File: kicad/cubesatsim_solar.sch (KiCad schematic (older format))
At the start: 23 parts, among them J1 Sensor Inputs, J10 INA219 Sensor Board, J11 INA219 Sensor Board, J12 INA219 Sensor Board, J13 3.5mm TRS Audio Jack with 2 S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, J14 RBF connector, J2 Battery In/Out, J3 Vdc In, J4 Vout to MoPOWER, J5 RBF Switch, J6 Expansion Interface, J7 INA219 Sensor Board, J8 INA219 Sensor Board, J9 INA219 Sensor Board, P3 Raspberry Pi GPIO Connector, U1 Variable Boost Converter Modu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

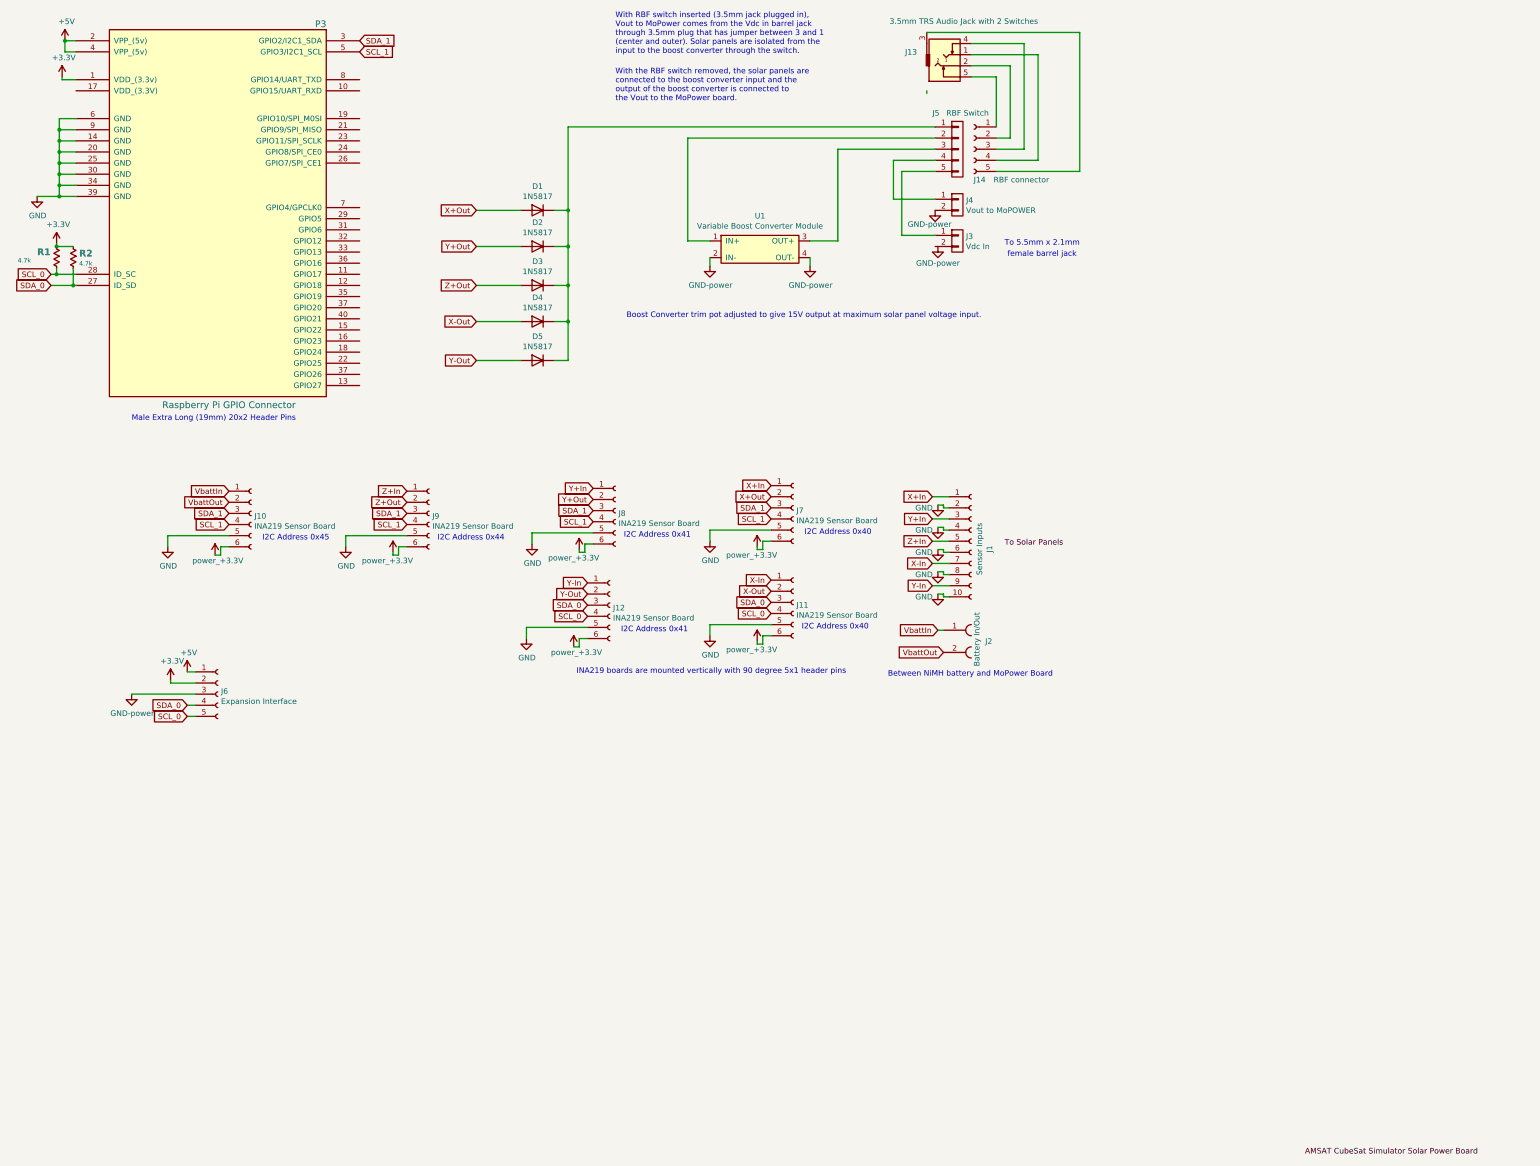
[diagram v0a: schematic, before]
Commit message: vB2 PCB Submitted to PCB Way
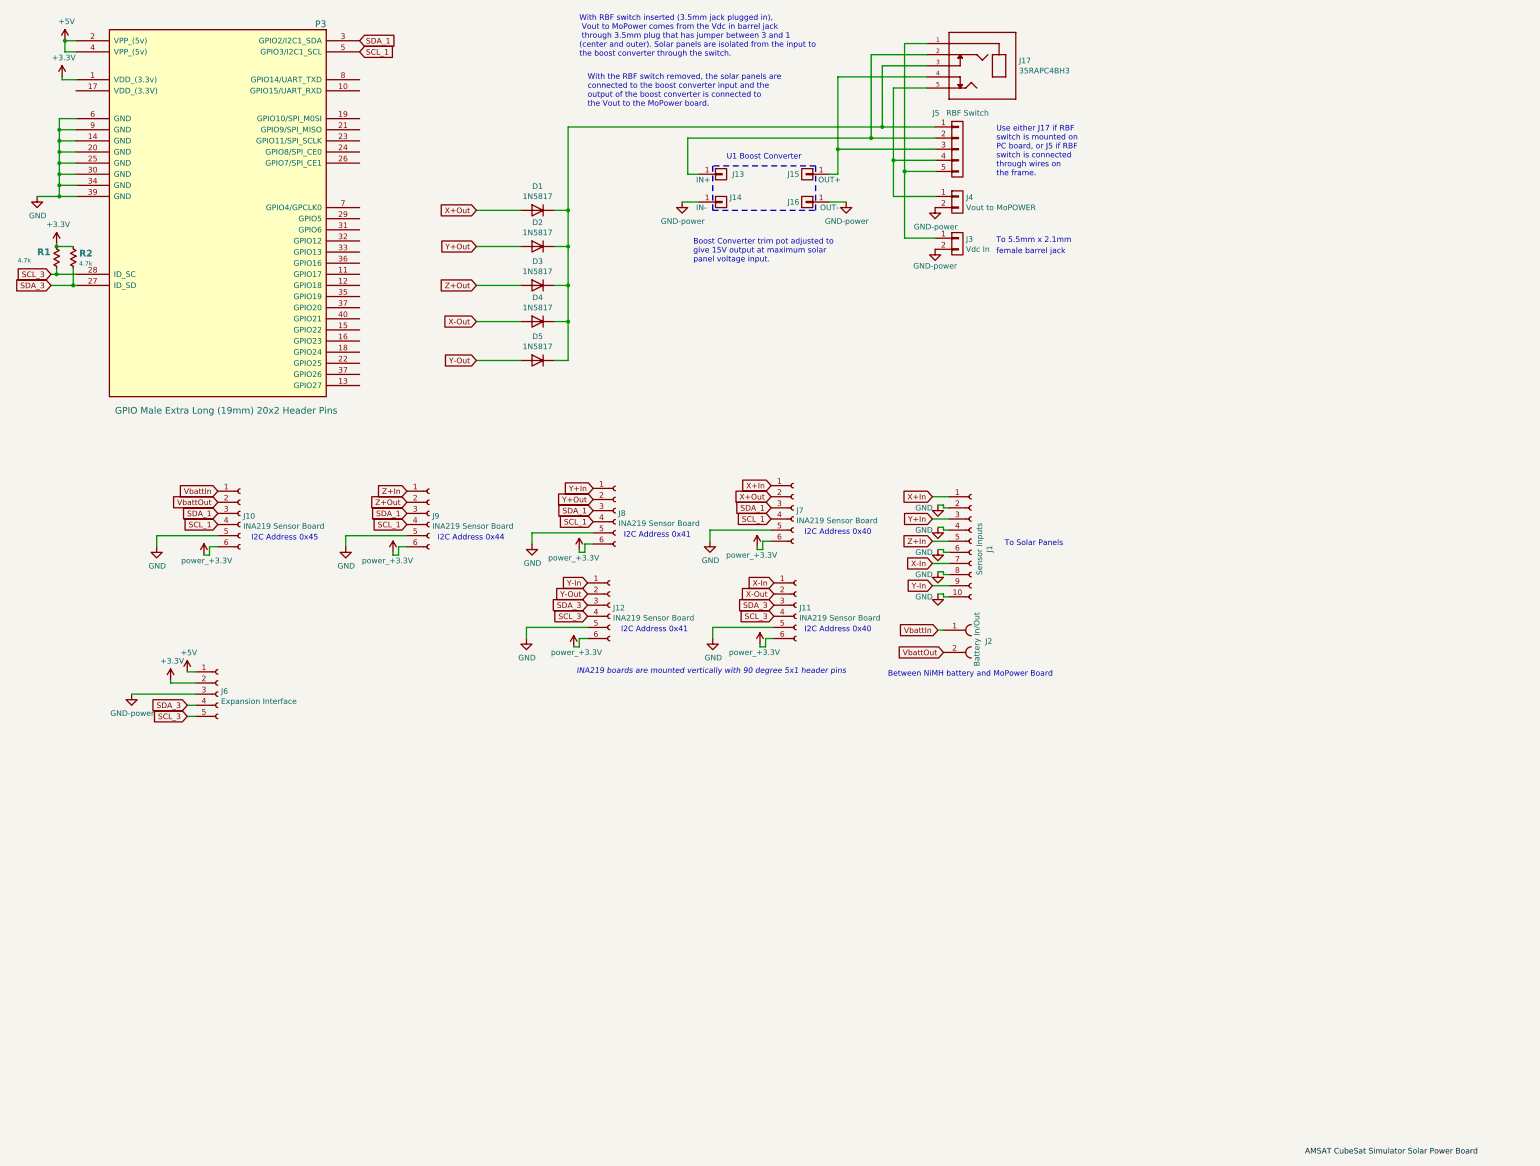
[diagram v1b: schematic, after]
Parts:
- removed J13: 3.5mm TRS Audio Jack with 2 Switches, symbol pihat_template-rescue:Audio-Jack-3_2Switches-conn2
- removed J14: RBF connector, symbol pihat_template-rescue:Conn_01x05_Female-Connector
- removed U1: Variable Boost Converter Module, symbol pihat_template-rescue:BoostConverter-New_Library
- added J13: IN+, Connector_PinSocket_2.54mm:PinSocket_1x01_P2.54mm_Vertical, symbol pihat_template-rescue:CONN_01X01-conn2
- added J14: IN-, Connector_PinSocket_2.54mm:PinSocket_1x01_P2.54mm_Vertical, symbol pihat_template-rescue:CONN_01X01-conn2
- added J15: OUT+, Connector_PinSocket_2.54mm:PinSocket_1x01_P2.54mm_Vertical, symbol pihat_template-rescue:CONN_01X01-conn2
- added J16: OUT-, Connector_PinSocket_2.54mm:PinSocket_1x01_P2.54mm_Vertical, symbol pihat_template-rescue:CONN_01X01-conn2
- added J17: 35RAPC4BH3, 35RAPC4BH3:SWITCHCRAFT_35RAPC4BH3, symbol 35RAPC4BH3:35RAPC4BH3
- J3, J4: footprint Connector_PinHeader_2.54mm:PinHeader_1x02_P2.54mm_Vertical -> Connector_Wire:SolderWirePad_1x02_P3.81mm_Drill1.2mm
- P3: value Raspberry Pi GPIO Connector -> GPIO Male Extra Long (19mm) 20x2 Header Pins; footprint w_conn_strip:vasch_strip_20x2 -> Connector_PinHeader_2.54mm:PinHeader_2x20_P2.54mm_Vertical
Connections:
- net GND: now also J3.2 (P2), J14.1 (P1), J16.1 (P1)
- net at D1.1 (K), D2.1 (K), D3.1 (K)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: now also J17.3
- net at J5.2 (P2): now also J13.1 (P1), J17.2
- net at J5.3 (P3): now also J15.1 (P1), J17.4
- net at J4.1 (P1), J5.4 (P4): now also J17.5
- net at J3.1 (P1), J5.5 (P5): now also J17.1
- net SCL_0 renamed SCL_3
- net SDA_0 renamed SDA_3
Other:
- note added: "Boost Converter trim pot adjusted to \ngive 15V output at maximum solar \npanel voltage input."
- note added: "To Solar Panels"
- note added: "U1 Boost Converter"
- note added: "Use either J17 if RBF \nswitch is mounted on \nPC board, or J5 if RBF \nswitch is connected \nthrough wires on \nthe frame."
- note added: "With RBF switch inserted (3.5mm jack plugged in),\n Vout to MoPower comes from the Vdc in barrel jack\n through 3.5mm plug that has jumper between 3 and 1 \n(center and outer). Solar panels are isolated from the input to \nthe boost converter through the switch."
- note removed: "Boost Converter trim pot adjusted to give 15V output at maximum solar panel voltage input."
- note removed: "Male Extra Long (19mm) 20x2 Header Pins"
- note removed: "With RBF switch inserted (3.5mm jack plugged in), \nVout to MoPower comes from the Vdc in barrel jack\nthrough 3.5mm plug that has jumper between 3 and 1 \n(center and outer). Solar panels are isolated from the \ninput to the boost converter through the switch.\n"
- moved on the sheet: J10, J11, J3, J4

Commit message: kicad files for vB3 PCB
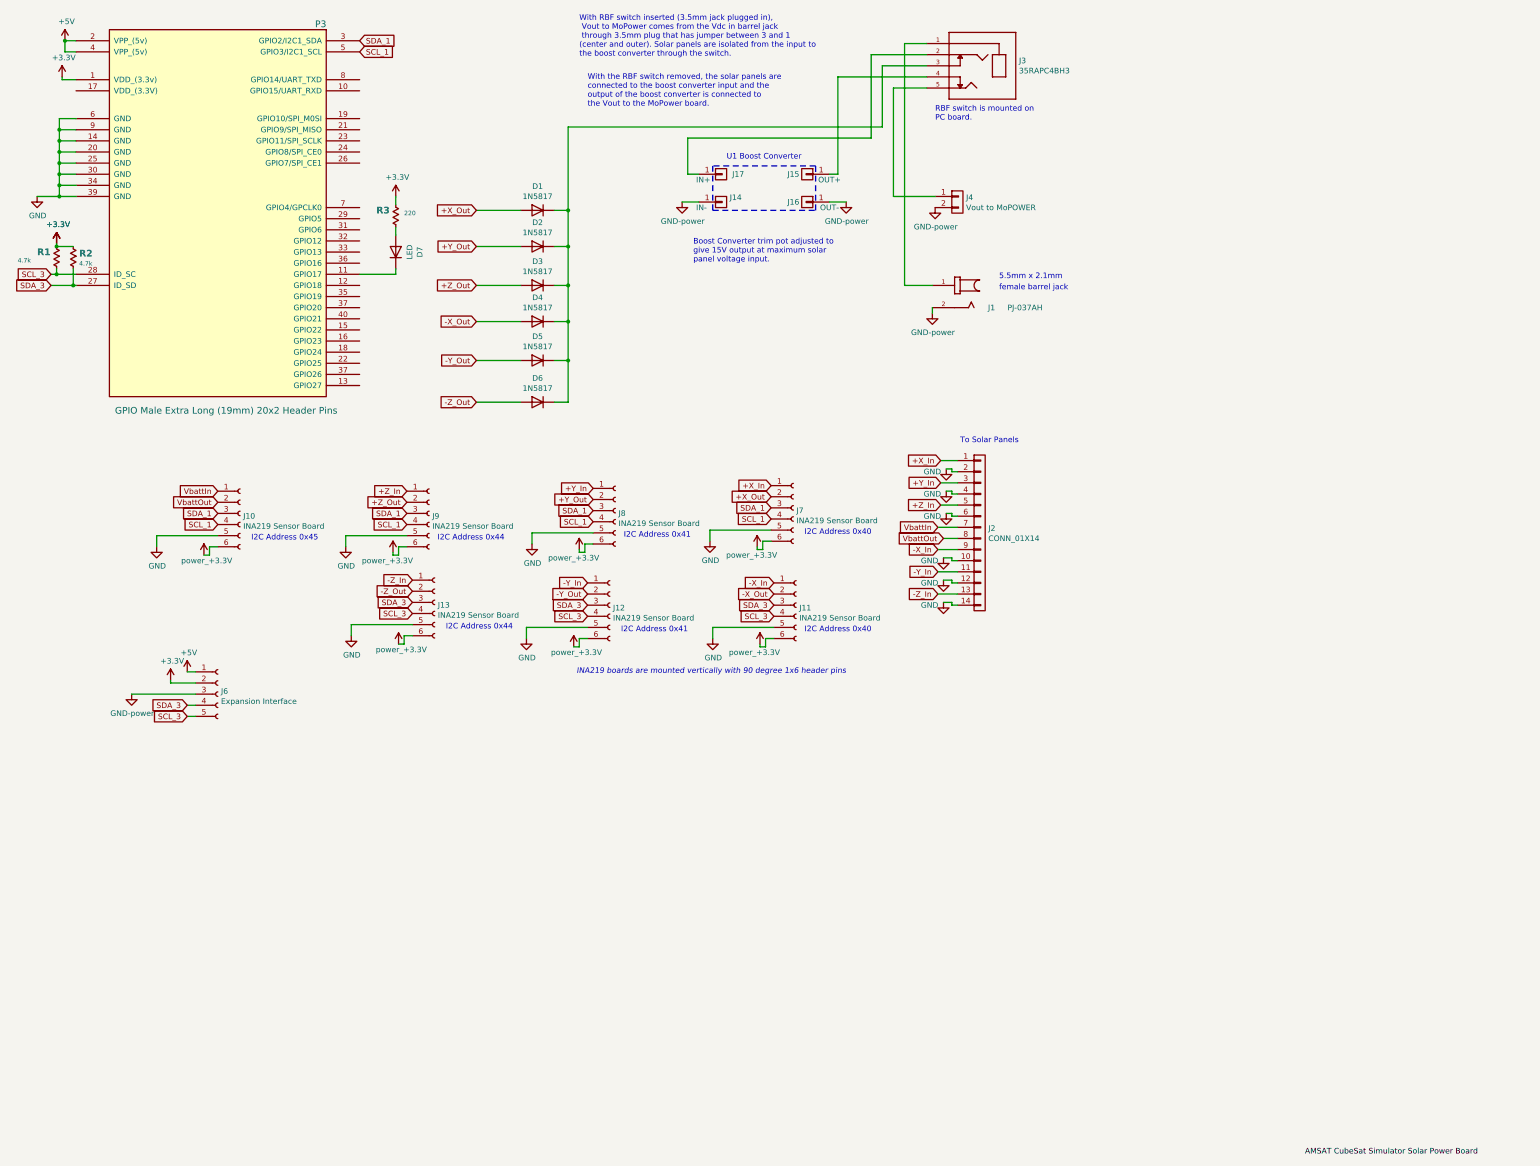
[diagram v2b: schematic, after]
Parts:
- removed J1: Sensor Inputs, Connector_PinHeader_2.54mm:PinHeader_1x10_P2.54mm_Vertical, symbol pihat_template-rescue:Conn_01x10_Female-Connector
- removed J2: Battery In/Out, Connector_PinHeader_2.54mm:PinHeader_1x02_P2.54mm_Vertical, symbol pihat_template-rescue:CONN_01X02_FEMALE-conn2
- removed J3: Vdc In, Connector_Wire:SolderWirePad_1x02_P3.81mm_Drill1.2mm, symbol pihat_template-rescue:CONN_01X02-conn2
- removed J5: RBF Switch, Connector_PinHeader_2.54mm:PinHeader_1x05_P2.54mm_Vertical, symbol pihat_template-rescue:CONN_01X05-conn2
- added D6: 1N5817, Diode_THT:D_DO-41_SOD81_P3.81mm_Vertical_AnodeUp, symbol pihat_template-rescue:D-device
- added D7: LED, Diode_THT:D_DO-41_SOD81_P3.81mm_Vertical_AnodeUp, symbol pihat_template-rescue:D-device
- added J1: PJ-037AH, PJ-037AH:CUI_PJ-037AH, symbol PJ-037AH:PJ-037AH
- added J13: INA219 Sensor Board, Connector_PinHeader_2.54mm:PinHeader_1x06_P2.54mm_Vertical, symbol pihat_template-rescue:Conn_01x06_Female-Connector
- added J2: CONN_01X14, Connector_PinSocket_2.54mm:PinSocket_1x14_P2.54mm_Vertical, symbol conn2:CONN_01X14
- added R3: 220, Resistor_THT:R_Axial_DIN0207_L6.3mm_D2.5mm_P5.08mm_Vertical, symbol pihat_template-rescue:RESISTOR-passive
- J4: footprint Connector_Wire:SolderWirePad_1x02_P3.81mm_Drill1.2mm -> Connector_PinSocket_2.54mm:PinSocket_2x01_P2.54mm_Vertical
- renumbered J13 to J17, J17 to J3
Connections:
- net +3V3: now also J13.6 (Pin_6), R3.1
- net GND: now also J1.2, J13.5 (Pin_5), J2.10 (P10), J2.12 (P12), J2.14 (P14), J2.2 (P2), J2.4 (P4), J2.6 (P6)
- net SCL_3: now also J13.4 (Pin_4)
- net SDA_3: now also J13.3 (Pin_3)
- net VbattIn: now also J2.7 (P7)
- net VbattOut: now also J2.8 (P8)
- net at P3.11 (GPIO17): now also D7.1 (K)
- net at D1.1 (K), D2.1 (K), D3.1 (K)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: now also D6.1 (K)
- net at J3.1: now also J1.1
- net X+In renamed +X_In
- net +X_In: now also J2.1 (P1)
- net X+Out renamed +X_Out
- net X-In renamed -X_In
- net -X_In: now also J2.9 (P9)
- net X-Out renamed -X_Out
- net Y+In renamed +Y_In
- net +Y_In: now also J2.3 (P3)
- net Y+Out renamed +Y_Out
- net Y-In renamed -Y_In
- net -Y_In: now also J2.11 (P11)
- net Y-Out renamed -Y_Out
- net Z+In renamed +Z_In
- net +Z_In: now also J2.5 (P5)
- net Z+Out renamed +Z_Out
- new net: D7.2 (A), R3.2
- new net -Z_In: J13.1 (Pin_1), J2.13 (P13)
- new net -Z_Out: D6.2 (A), J13.2 (Pin_2)
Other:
- note added: "5.5mm x 2.1mm"
- note added: "I2C Address 0x44"
- note added: "INA219 boards are mounted vertically with 90 degree 1x6 header pins"
- note added: "RBF switch is mounted on \nPC board.\n"
- note removed: "Between NiMH battery and MoPower Board"
- note removed: "INA219 boards are mounted vertically with 90 degree 5x1 header pins"
- note removed: "To 5.5mm x 2.1mm"
- note removed: "Use either J17 if RBF \nswitch is mounted on \nPC board, or J5 if RBF \nswitch is connected \nthrough wires on \nthe frame."
